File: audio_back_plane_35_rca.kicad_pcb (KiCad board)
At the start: 4 copper layers, 120 x 100 mm, 110 parts, among them J3 RCA-IN, J4 Conn_01x08, J6 RCA-OUT, U1 Teensy 4.1 - DEVKIT, U10 SN74LVC1T45DBV, U11 SN74LVC1T45DBV, U12 SN74LVC1T45DBV, U13 SN74LVC1T45DBV, U14 Single Buffer - 74LVC1G125GV,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, U15 Single Buffer - 74LVC1G125GV,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, U16 Single Buffer - 74LVC1G125GV,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, U2 ESP32-DevKitC - DEVKIT, U5 Optoisolators - H11L1SM - 6-S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, U6 Dual Buffer - 74HCT2G17GW,125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, U7 Single Buffer - 74LVC1G125GV,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, U8 Single Buffer - 74LVC1G125GV,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, U9 SN74LVC1T45DBV

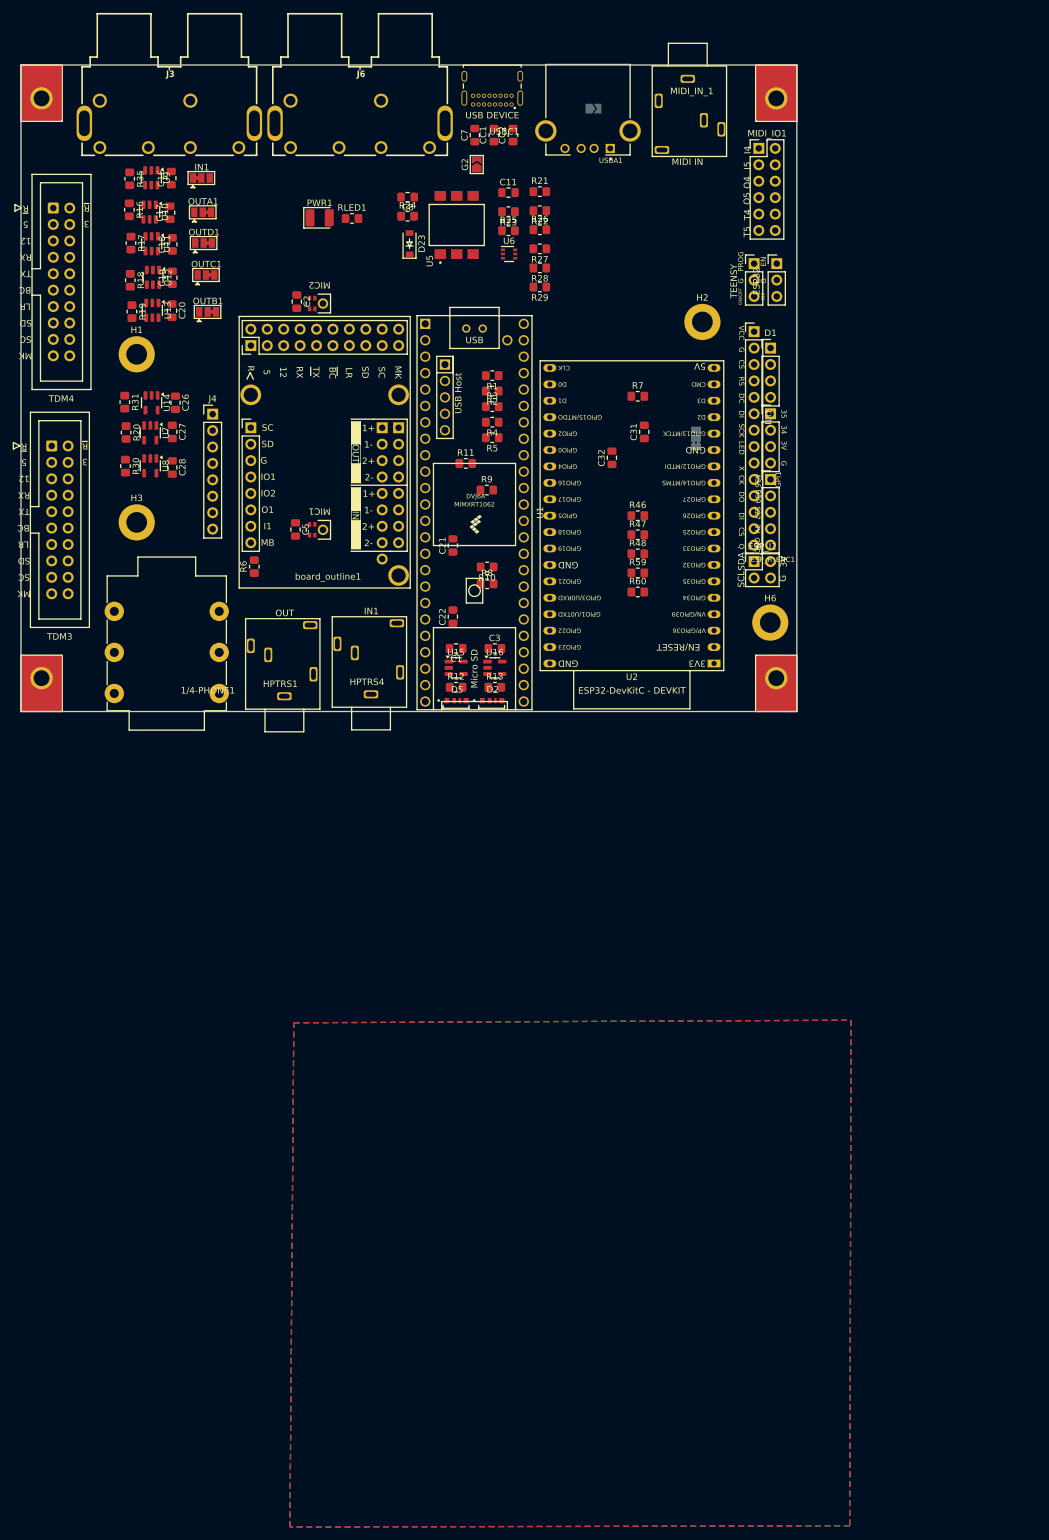
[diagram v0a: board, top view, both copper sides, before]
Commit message: update
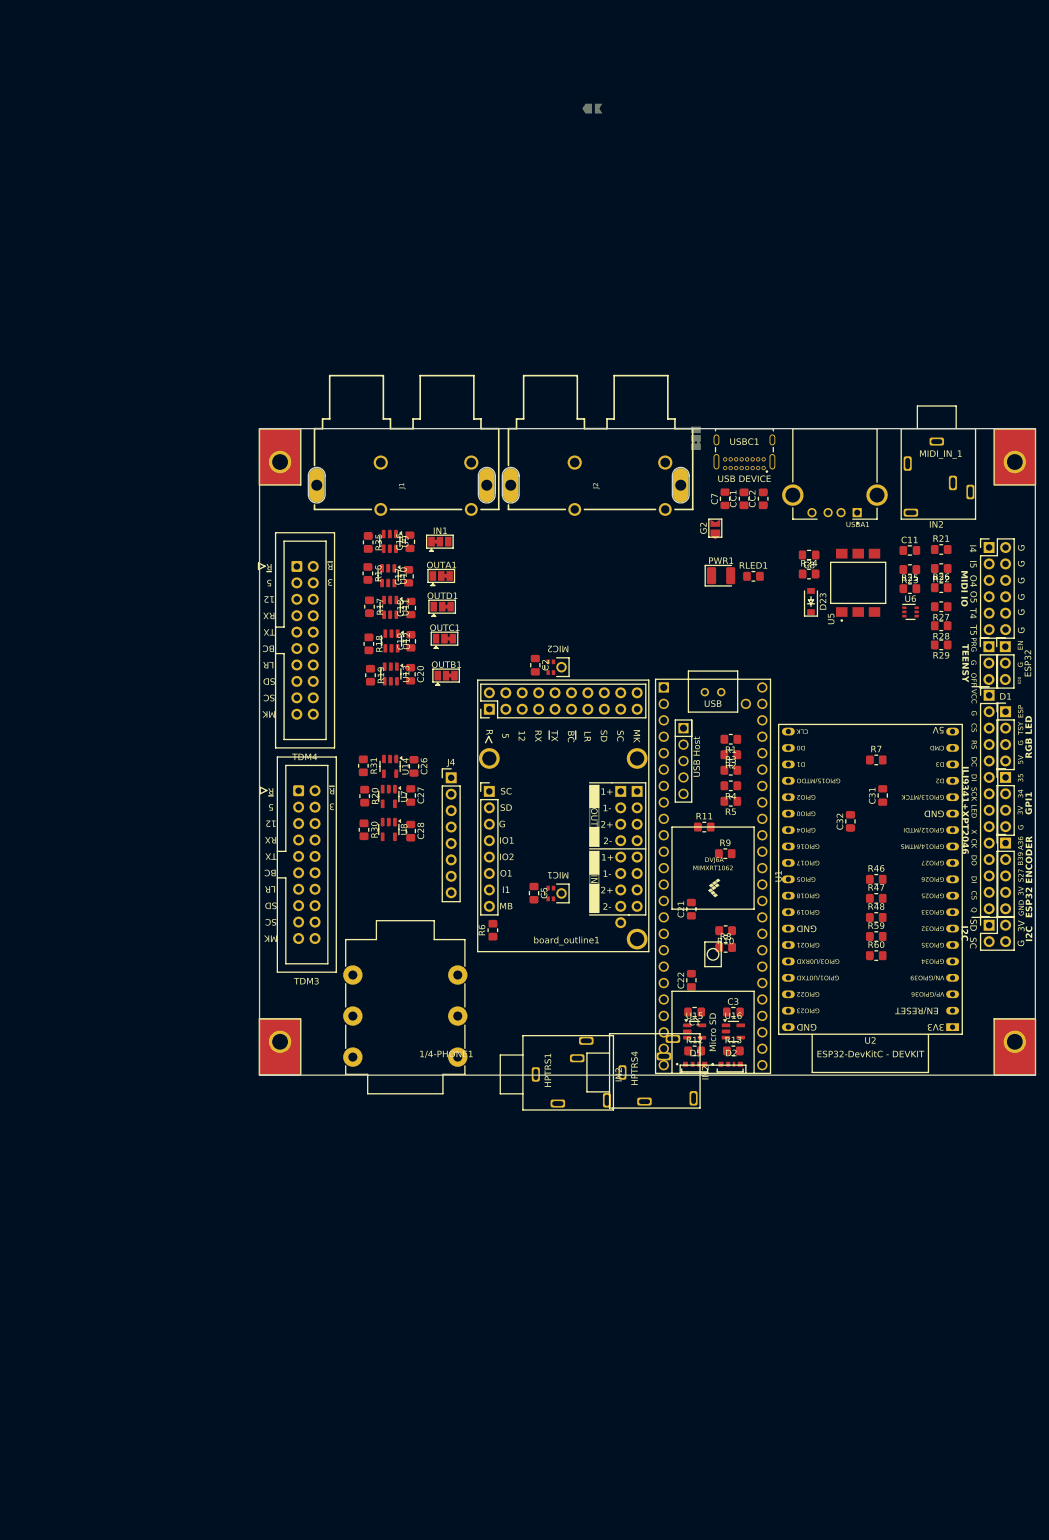
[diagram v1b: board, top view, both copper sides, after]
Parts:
- removed H1, H2, H3, H6: MountingHole_Pad, MountingHole:MountingHole_3.2mm_M3_DIN965_Pad
- removed J3: RCA-IN, project_fp:PJRAS2X1_NOT-VERIFIED
- removed J6: RCA-OUT, project_fp:PJRAS2X1_NOT-VERIFIED
- added J1: PJRAS2X1S01X, project_fp:PJRAS2X1S01X_MOD2, F.Cu at (122.0, 100.0)
- added J2: PJRAS2X1S01X, project_fp:PJRAS2X1S01X_MOD2, F.Cu at (152.0, 100.0)
- D1: footprint project_fp:PinHeader_1x04_P2.54mm_Vertical -> project_fp:LED_GPIO_PinHeader_1x04_P2.54mm_Vertical
- moved board_outline2 93.9 mm to (100.0, 100.0), turned to -90 degrees
- moved PWR1 83.2 mm to (171.4, 122.7)
- moved RLED1 83.2 mm to (176.4, 122.8)
- moved C8 83.2 mm to (185.0, 119.5)
- moved D23 83.2 mm to (185.3, 126.7)
- moved R23 83.2 mm to (200.6, 121.8)
- moved R24 83.2 mm to (185.0, 122.5)
- moved R25 83.2 mm to (200.6, 124.7)
- moved R26 83.2 mm to (205.4, 124.6)
- moved R27 83.2 mm to (205.4, 127.5)
- moved R28 83.2 mm to (205.4, 130.5)
- moved U5 83.2 mm to (192.6, 123.9)
- moved U6 83.2 mm to (200.7, 128.3)
- moved C11 83.2 mm to (200.6, 118.8)
- moved R21 83.2 mm to (205.4, 118.7)
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- renumbered T_PROG2 to ESP_PROG1
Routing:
- removed copper zone on B.Cu, net GND
- removed copper zone on F.Cu, net GND
- removed copper zone on In1.Cu, net GND
- removed copper zone on In2.Cu, net GND
